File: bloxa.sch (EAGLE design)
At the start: 93 parts, among them CON1 CON-4P-JST_GH-RA, CON2 CON-4P-JST_GH-RA, IC1 MCP9700-SC70-5, IC2 TPD3S014DBVR-SOT23-6, IC3 TJA1051(X)/3-SO8, J1 CONNECTION, J2 CONNECTION, Q1 BUK9K6R2-40E,115, Q2 BUK9K6R2-40E,115, Q3 BUK9K6R2-40E,115

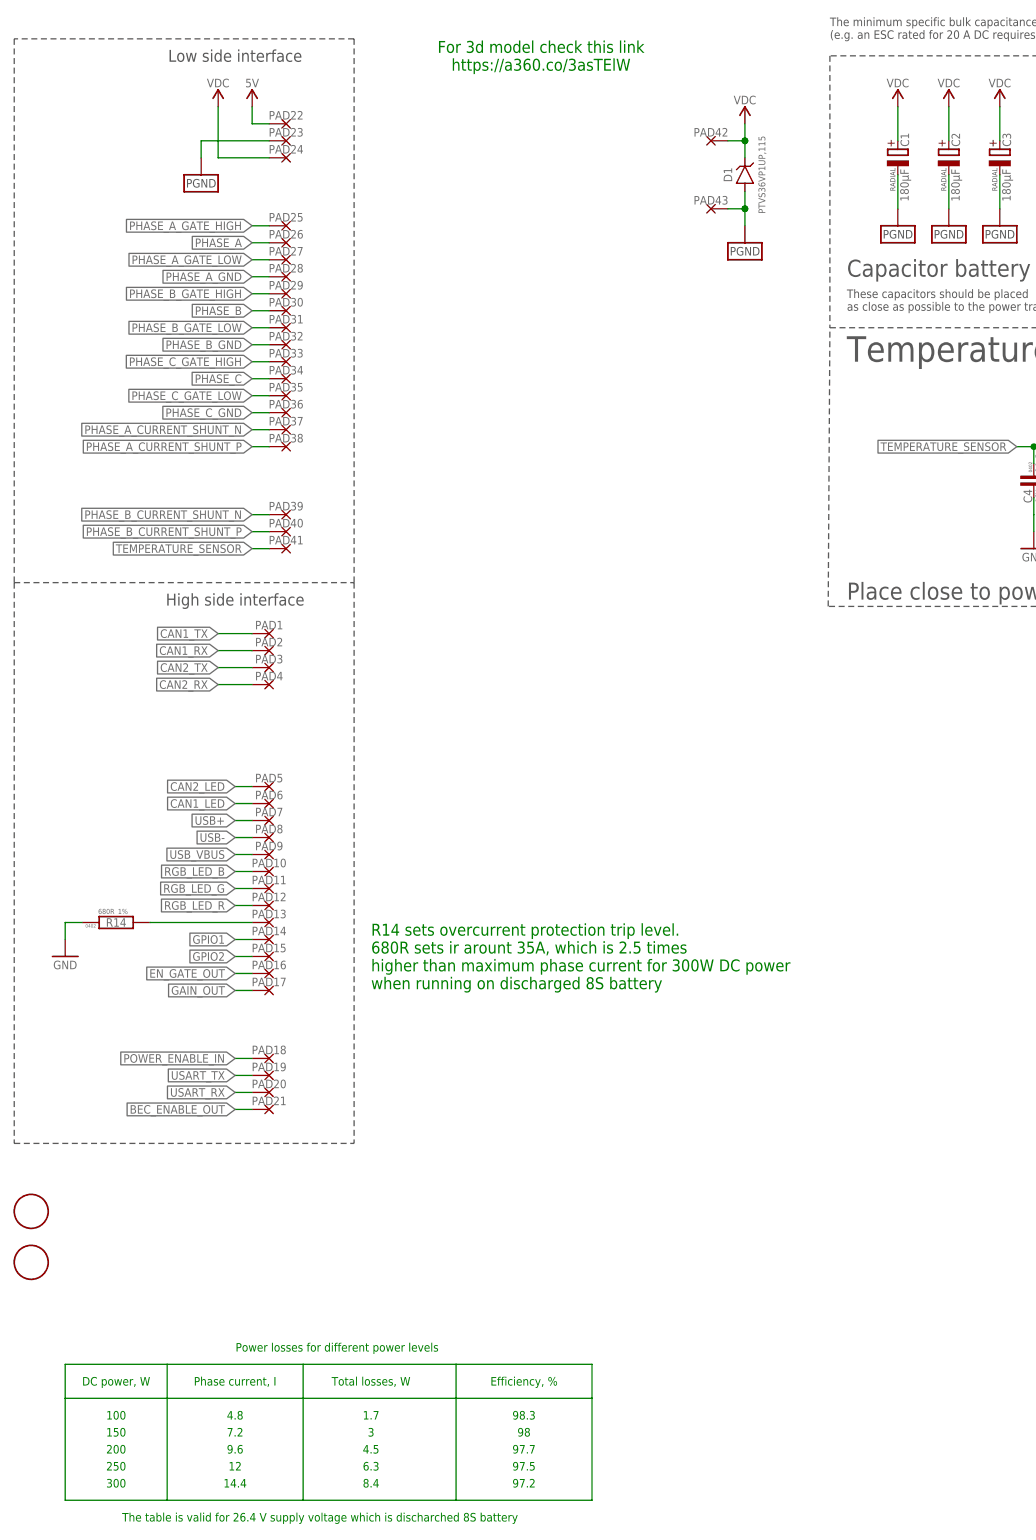
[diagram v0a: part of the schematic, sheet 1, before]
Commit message: ERC re-check
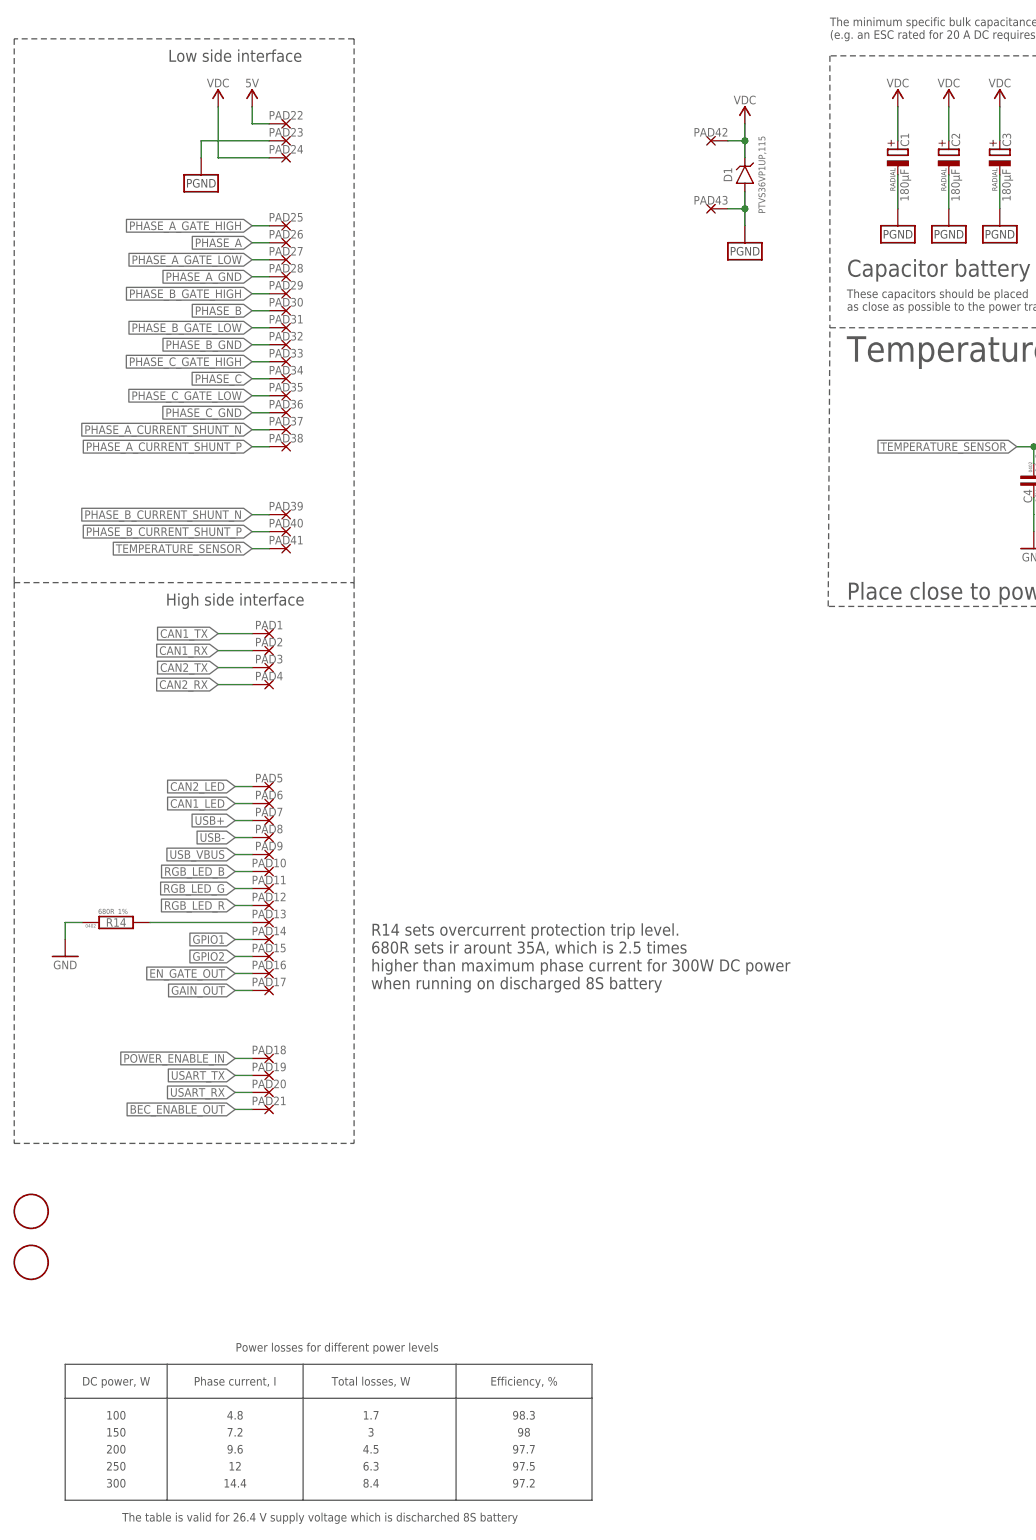
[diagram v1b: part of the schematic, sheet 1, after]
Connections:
- removed net N$2: IC3.S
- net GND: now also IC3.S
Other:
- note removed: "For 3d model check this link https://a360.co/3asTElW"
